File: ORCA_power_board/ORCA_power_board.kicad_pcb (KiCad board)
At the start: 4 copper layers, 73 x 86.2 mm, 132 parts, among them J1 data_line_power, J2 I2C_power, J21 Conn_01x02, J3 Vout_motor, J4 emergence, J5 Vin_batt, J6 Vin_ex, J7 Vout_power2usp, J8 Vin_power2usp, J9 +5Vout_cpu, Q1 TJ60S04M3L, Q2 BSS138, Q3 BSS138, Q4 BSS138, Q5 TJ60S04M3L, U1 LTC2301IMS, U10 HY2112, U11 AP64502, U12 TPS61230A__board, U2 NJM78055DL1, U3 CN3058E, U4 RH1B-UDC6V, U5 TPH11006NL, U6 TPH11006NL, U7 NJW4860, U8 AZ1117-3.3, U9 FS8205

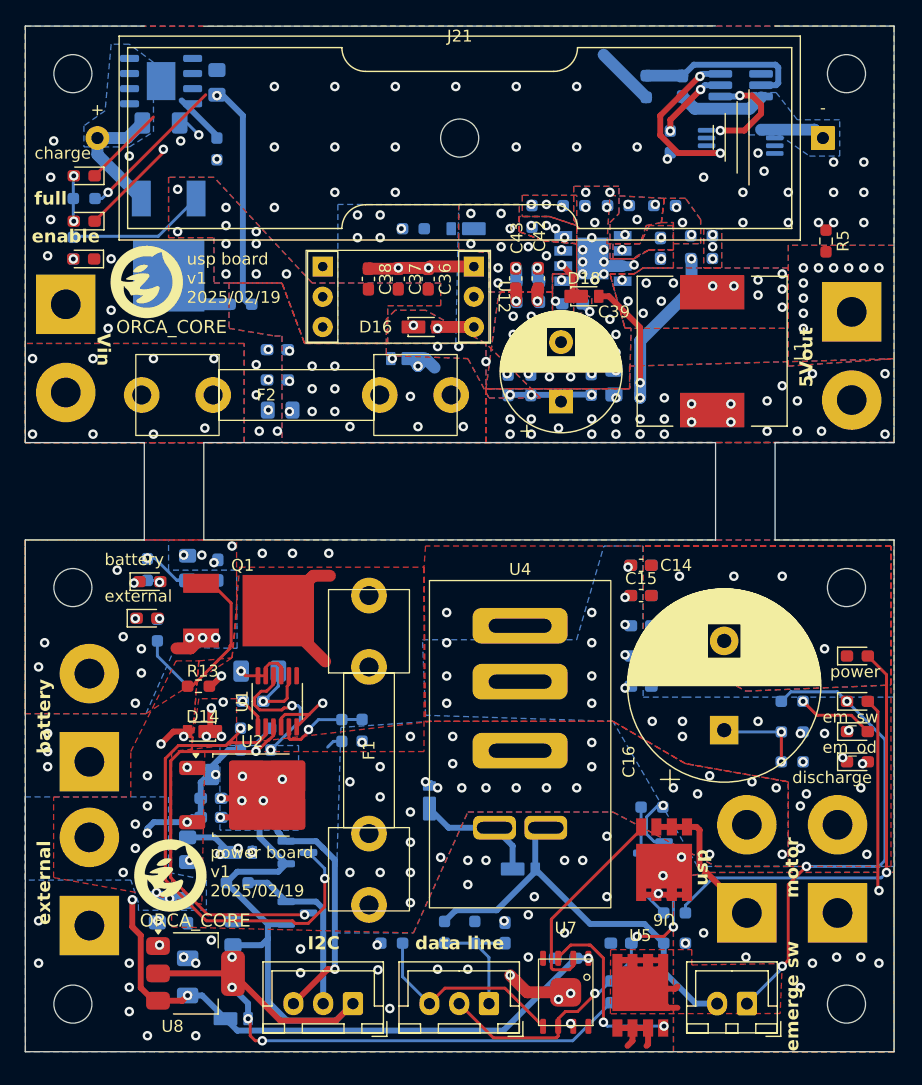
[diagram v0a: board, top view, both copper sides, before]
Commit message: complete power_board
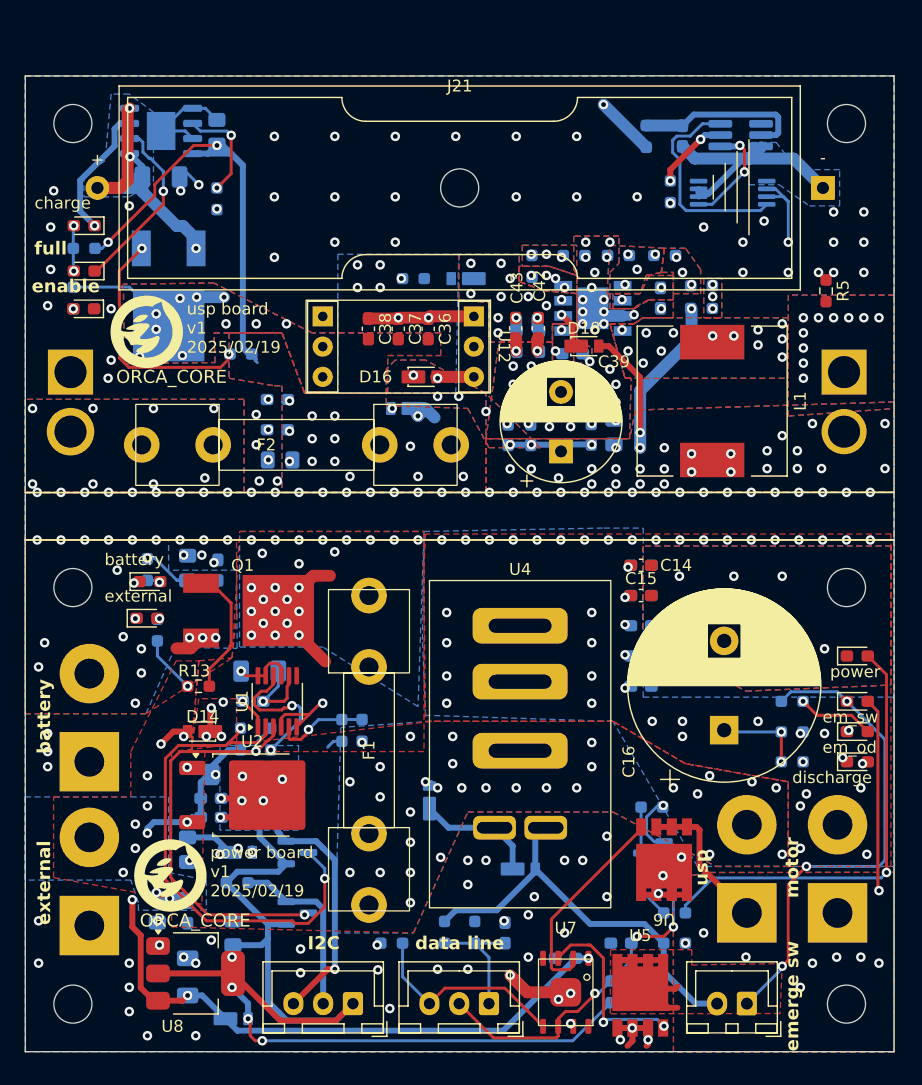
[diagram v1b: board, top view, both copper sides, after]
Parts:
- J8: footprint Conn:power_pad -> Conn:AMASS_XT30U-F_Vertical_withmodel_female; moved to B.Cu
- J9: footprint Conn:power_pad -> Conn:AMASS_XT30U-F_Vertical_withmodel_male; moved to B.Cu
- U9: value FS8205 -> FS8205A
- moved C25 4.54 mm to (116.6, 66.8)
- moved J8 4.52 mm to (109.1, 85.8)
- moved U9 4.33 mm to (164.6, 68.1)
- moved D10 4.19 mm to (110.2, 70.9)
- moved ORCA_CORE 4.19 mm to (115.6, 79.8)
- moved Q5 4.19 mm to (117.2, 76.3)
- moved R22 4.19 mm to (110.1, 72.8)
- moved R24 4.19 mm to (151.3, 73.4)
- moved R27 4.19 mm to (158.9, 73.4)
- moved R28 4.19 mm to (155.0, 73.4)
- moved R33 4.19 mm to (123.3, 81.7)
- moved C35 4.19 mm to (160.4, 63.4)
- moved R30 4.19 mm to (157.4, 63.4)
- moved U10 4.19 mm to (165.3, 63.3)
- moved C24 4.19 mm to (121.3, 63.0)
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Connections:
- Q5 pad 1: batt+ -> reg_up
- Q5 pad 3: reg_up -> batt+
- U3 pad 9: (no net) -> GND
- U9 pad 1: batt- -> unconnected-(U9-Pad1)
- U9 pad 2: unconnected-(U9-Pad2) -> GND
- U9 pad 5: unconnected-(U9-Pad5) -> Net-(U10-OD)
- U9 pad 6: Net-(U10-OD) -> batt-
- U9 pad 7: (no net) -> batt-
- U9 pad 8: (no net) -> unconnected-(U9-Pad8)
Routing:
- net batt+: track 16.0 -> 82.0 mm, vias 0 -> 4
- net Net-(Q5-G): track 6.14 -> 20.4 mm, vias 0 -> 2
- net GND: track 65.2 -> 75.5 mm, vias 161 -> 181
- net batt-: track 12.9 -> 20.6 mm
- net +VDD_usp: track 34.8 -> 42.4 mm
- net Net-(D12-K): track 8.43 -> 15.3 mm
- net +VDD_power: track 16.1 -> 10.6 mm
- net Net-(U3-ISET): track 4.39 -> 8.77 mm, vias 0 -> 2
- net Net-(D10-K): track 6.99 -> 11.3 mm, vias 0 -> 1
- net Net-(U10-OC): track 13.8 -> 17.9 mm, vias 2 -> 0
- net reg_up: track 11.7 -> 13.7 mm
- net Net-(Q1-G): track 12.0 -> 11.1 mm
- net reg_down_out: vias 38 -> 53
- net Net-(D14-K): vias 4 -> 28
- net /usp/Vin: vias 8 -> 17
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- added copper zone on B.Cu, net Net-(D14-K)
- added copper zone on In2.Cu, net Net-(D14-K)
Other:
- board size 73 x 86.2 mm -> 73 x 82 mm
